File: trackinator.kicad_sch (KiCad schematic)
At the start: 2 parts, among them U6 FE2.1

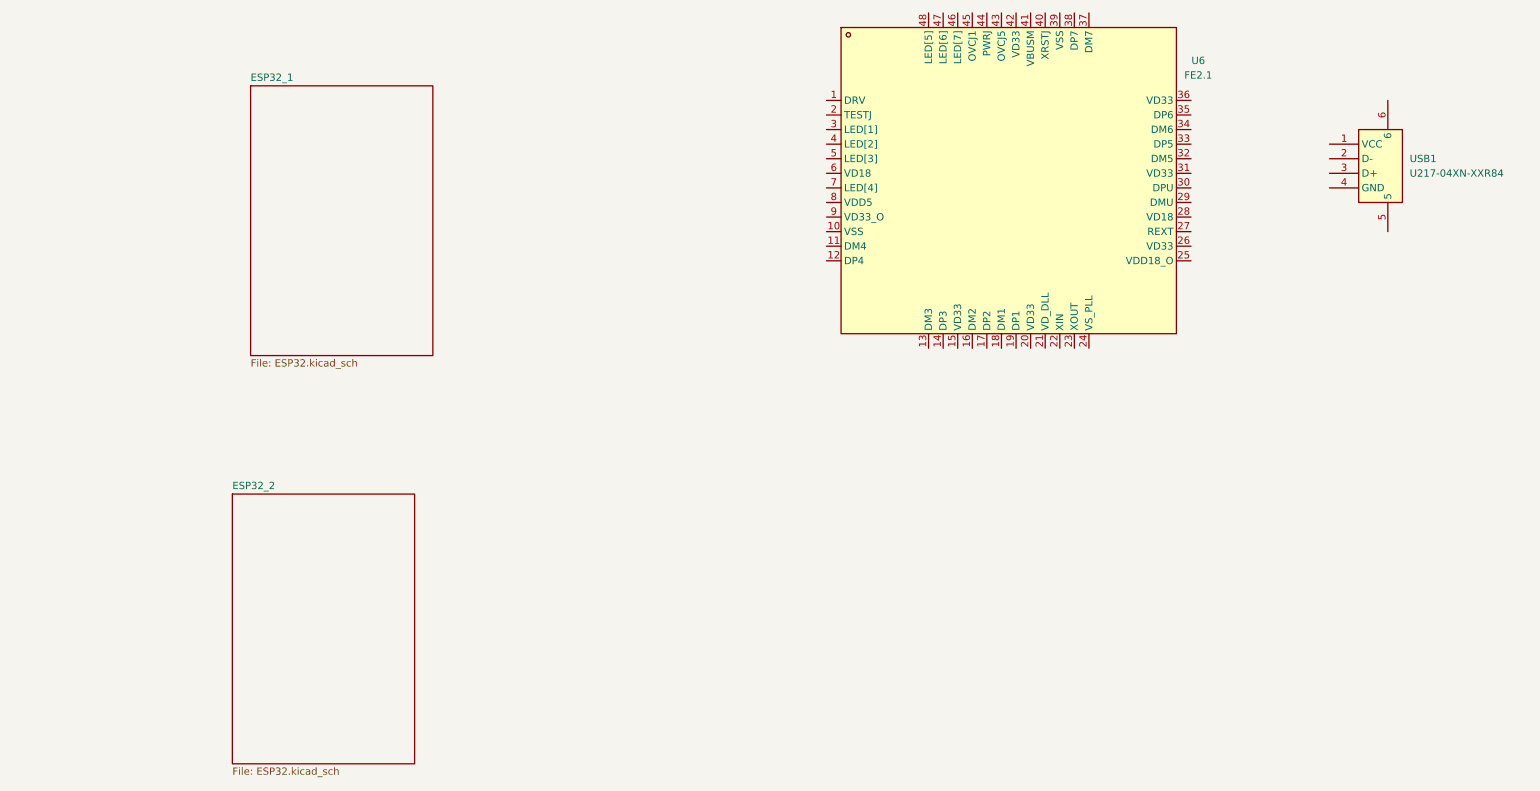
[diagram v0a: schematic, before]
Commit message: revving up
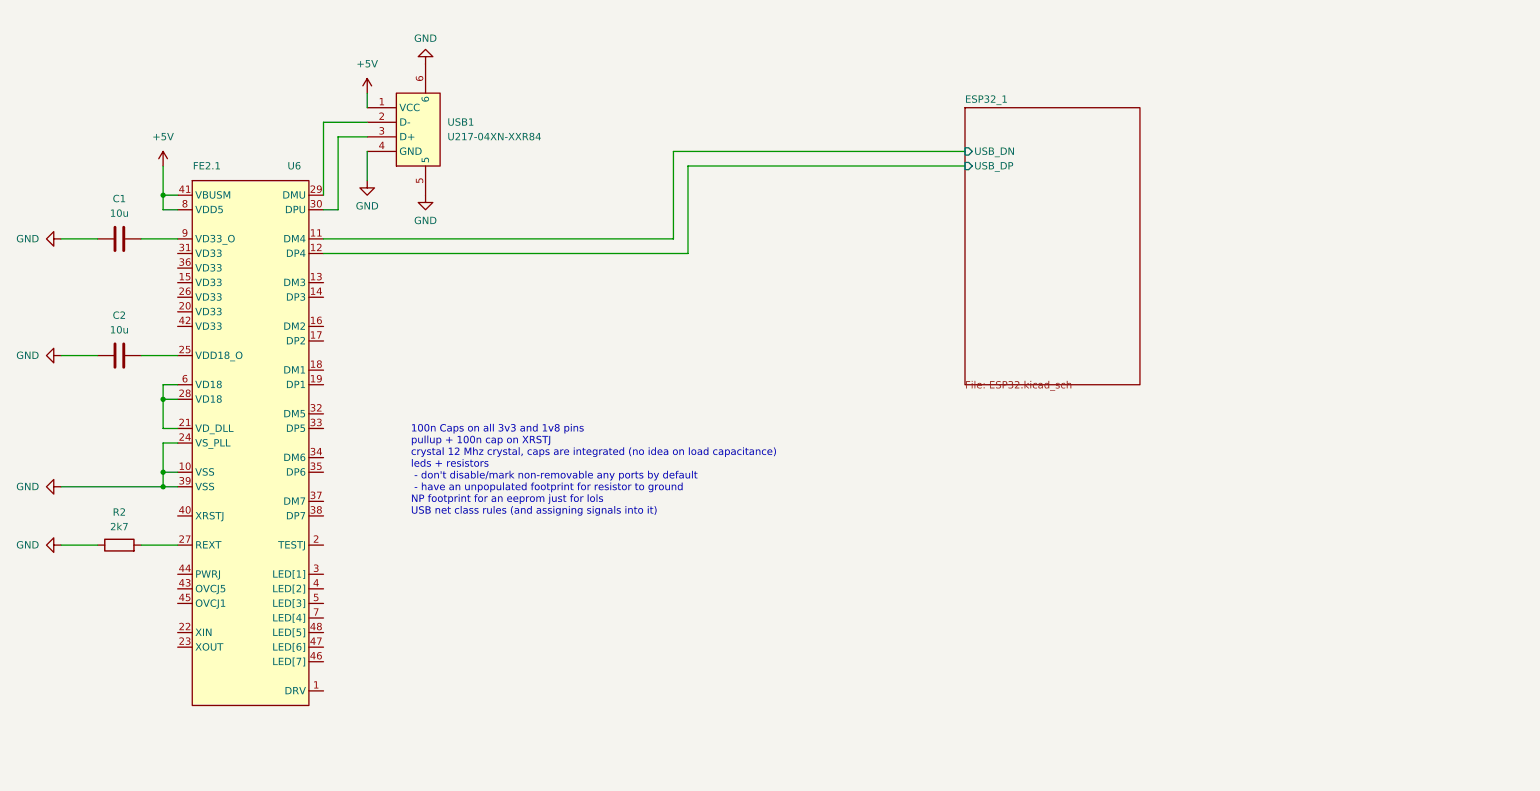
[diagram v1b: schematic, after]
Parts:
- added C1, C2: 10u, symbol Device:C
- added R2: 2k7, symbol Device:R
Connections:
- net GND: now reaches U6.10 (VSS)
- net GND: now also U6.24 (VS_PLL), U6.39 (VSS), USB1.4 (GND), USB1.5, USB1.6, C1.1, C2.1, R2.1
- net ESP32_1/USB_DN: now reaches U6.11 (DM4)
- net ESP32_1/USB_DP: now reaches U6.12 (DP4)
- net at U6.21 (VD_DLL): now also U6.28 (VD18), U6.6 (VD18)
- net at U6.25 (VDD18_O): now also C2.2
- net at U6.27 (REXT): now also R2.2
- net at U6.29 (DMU): now also USB1.2 (D-)
- net at U6.30 (DPU): now also USB1.3 (D+)
- net +5V: now reaches U6.41 (VBUSM)
- net +5V: now also U6.8 (VDD5), USB1.1 (VCC)
- net at U6.9 (VD33_O): now also C1.2
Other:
- removed sheet ESP32_2
- sheet ESP32_1 ports: added USB_DN, USB_DP; removed none
- note added: "100n Caps on all 3v3 and 1v8 pins pullup + 100n cap on XRSTJ crystal 12 Mhz crystal, caps are integrated (no idea on load capacitance) leds + resistors - don't disable/mark non-removable any ports by default - have an unpopulated footprint for resistor to ground NP footprint for an eeprom just for lols USB net class rules (and assigning signals into it)"
- moved on the sheet: USB1
